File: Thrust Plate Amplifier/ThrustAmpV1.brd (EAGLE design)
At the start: 130.8 x 78.7 mm, 54 parts, among them U1 INA126PA, U2 INA126PA, U3 INA126PA, U4 INA126PA, U5 LP2985AIM5-3.3, U6 LP2985AIM5-5.0/NOPB

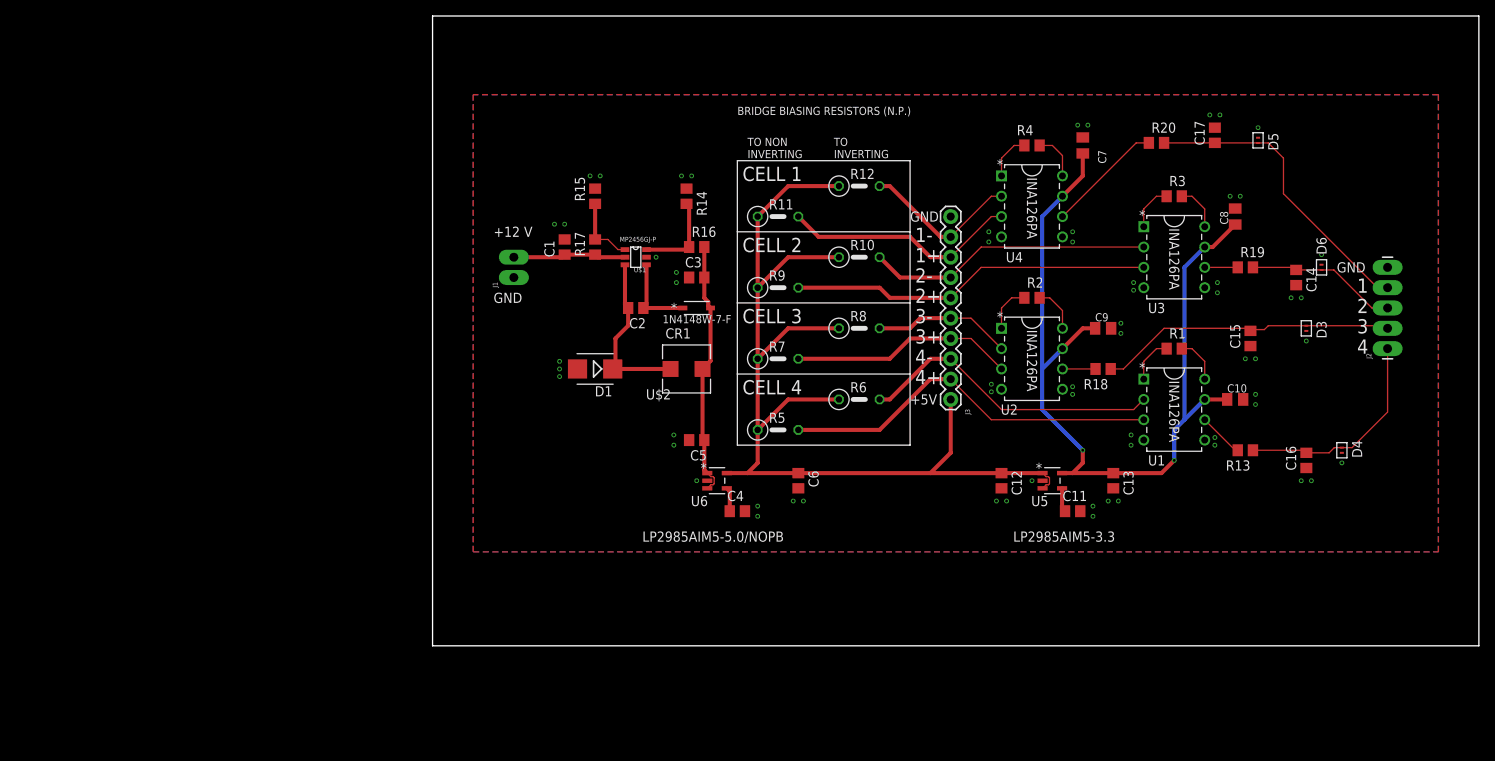
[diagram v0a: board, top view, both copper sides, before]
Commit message: Major layout changes, per design review
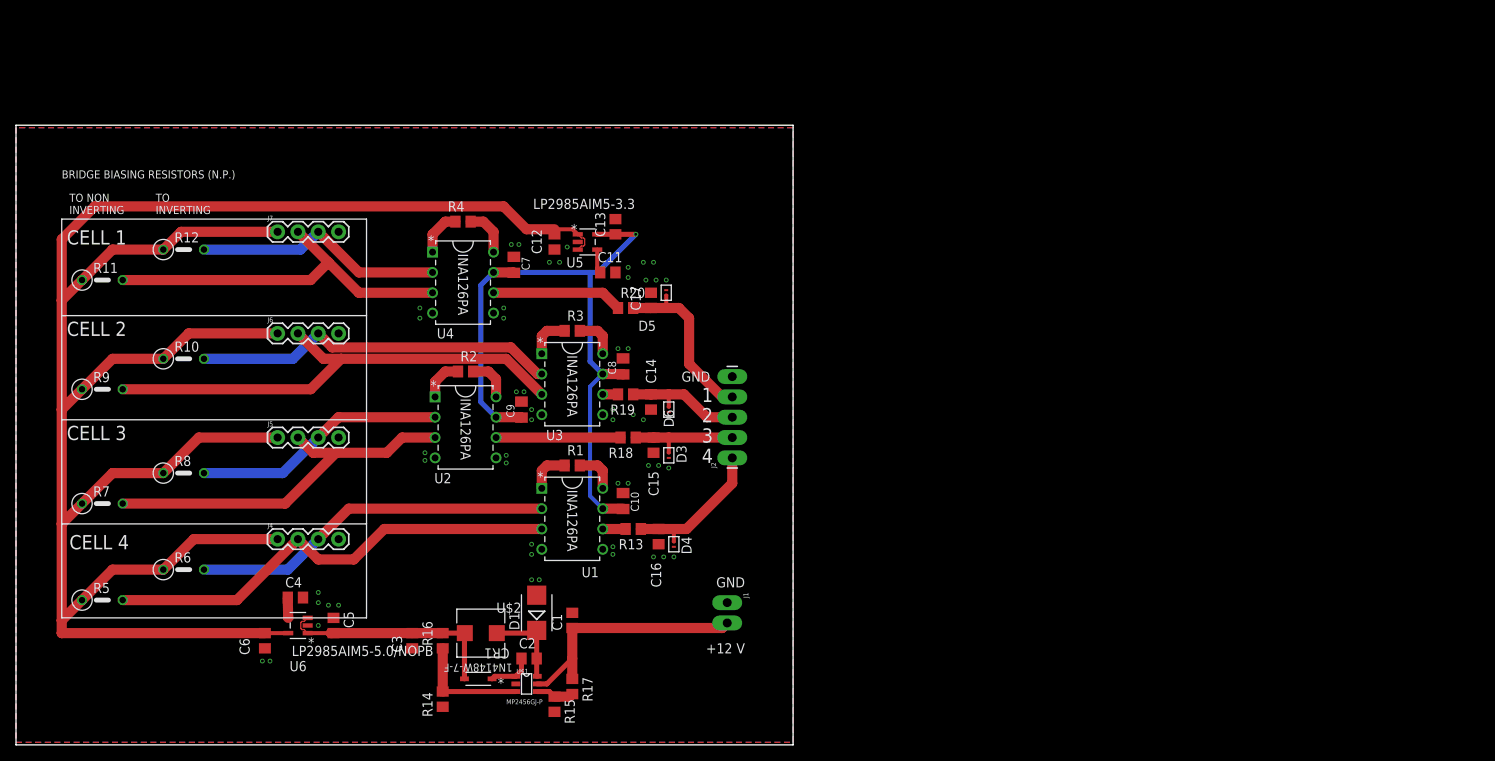
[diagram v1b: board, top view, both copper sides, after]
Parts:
- removed J3: (no value), SparkFun-Connectors:1X10
- added J4, J5, J6, J7: (no value), SparkFun-Connectors:1X04
- C13, C6: value 2,2 uF -> 2.2 uF
- R1, R2, R3, R4: value (none) -> TBD
- moved R5 87.1 mm to (10.8, 18.1)
- moved R6 87.1 mm to (21.0, 21.9)
- moved R7 86.4 mm to (10.8, 30.2)
- moved R8 86.4 mm to (21.0, 34.0)
- moved R10 85.4 mm to (21.0, 48.3)
- moved R9 85.4 mm to (10.8, 44.5)
- moved R11 84.8 mm to (10.8, 58.1)
- moved R12 84.8 mm to (21.0, 61.9)
- moved D4 84.3 mm to (82.2, 25.1)
- moved D6 83.5 mm to (81.6, 41.9), turned to 0 degrees
- moved J2 83.0 mm to (89.5, 35.9)
- moved C14 82.1 mm to (79.4, 42.9)
- moved C16 81.5 mm to (80.3, 26.0)
- moved D3 81.3 mm to (81.6, 36.2)
- moved R19 79.1 mm to (76.2, 43.8)
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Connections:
- removed net N$14: J3.2, R5.2, U1.3
- removed net N$15: J3.5, R8.2, U2.2
- removed net N$16: J3.4, R7.2, U2.3
- removed net N$29: J3.3, R6.2, U1.2
- removed net N$32: J3.6, R9.2, U3.3
- removed net N$33: J3.7, R10.2, U3.2
- removed net N$34: J3.8, R11.2, U4.3
- removed net N$35: J3.9, R12.2, U4.2
- new net 0: J1.1
- new net N$100: J7.3, R12.2, U4.2
- new net N$93: J4.2, R5.2, U1.3
- new net N$94: J4.3, R6.2, U1.2
- new net N$95: J5.2, R7.2, U2.3
- new net N$96: J5.3, R8.2, U2.2
- new net N$97: J6.2, R9.2, U3.3
- new net N$98: J6.3, R10.2, U3.2
- new net N$99: J7.2, R11.2, U4.3
- net 5V: now also J4.1, J5.1, J6.1, J7.1; no longer J3.1
- net GND: now also J4.4, J5.4, J6.4, J7.4; no longer J1.1, J3.10
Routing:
- net 5V: track 132.2 -> 272.9 mm
- net N$97: track 0.00 -> 62.5 mm
- net N$93: track 0.00 -> 58.2 mm
- net N$95: track 0.00 -> 48.0 mm
- net N$14: track 47.9 -> 0.00 mm
- net N$99: track 0.00 -> 46.6 mm
- net N$98: track 0.00 -> 45.6 mm
- net N$94: track 0.00 -> 45.4 mm
- net N$32: track 45.3 -> 0.00 mm
- net N$29: track 38.3 -> 0.00 mm
- net N$33: track 35.7 -> 0.00 mm
- net N$96: track 0.00 -> 31.8 mm
- net N$100: track 0.00 -> 31.6 mm
- net N$34: track 29.6 -> 0.00 mm
- net N$16: track 28.0 -> 0.00 mm
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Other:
- board size 130.8 x 78.7 mm -> 97.1 x 77.5 mm
- board text removed: "+5V"
- board text removed: "1+"
- board text removed: "1-"
- board text removed: "2+"
- board text removed: "2-"
- board text removed: "3+"
- board text removed: "3-"
- board text removed: "4+"
- board text removed: "4-"
